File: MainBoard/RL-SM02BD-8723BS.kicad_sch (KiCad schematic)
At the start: 20 parts, among them U401 RTL8723BS(ComboModule)

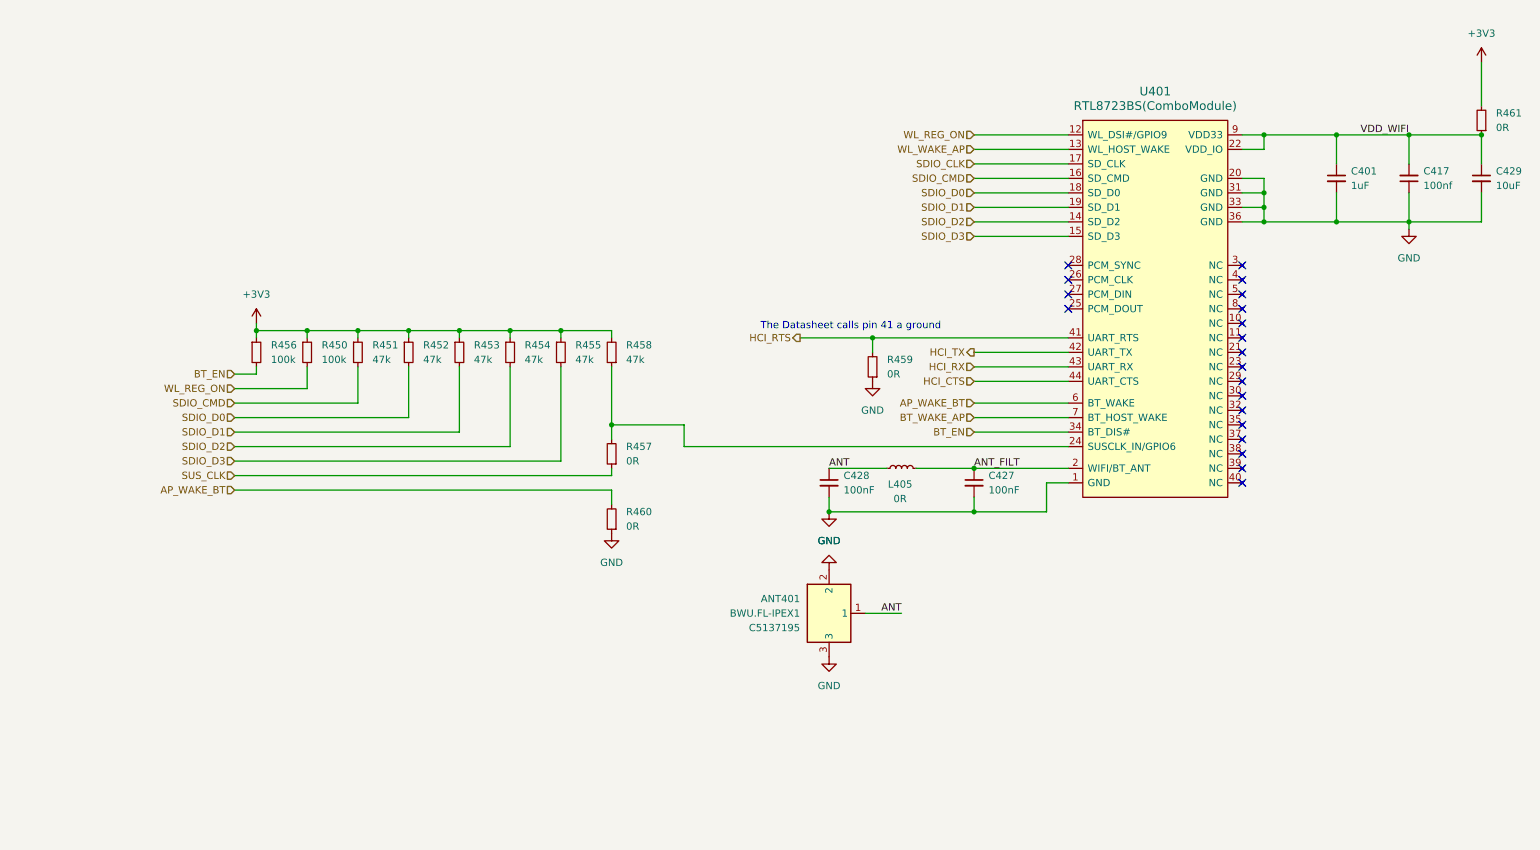
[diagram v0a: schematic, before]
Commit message: Submit for fab rev 2
Signed-off-by: Connor Rigby <connorr@hey.com>
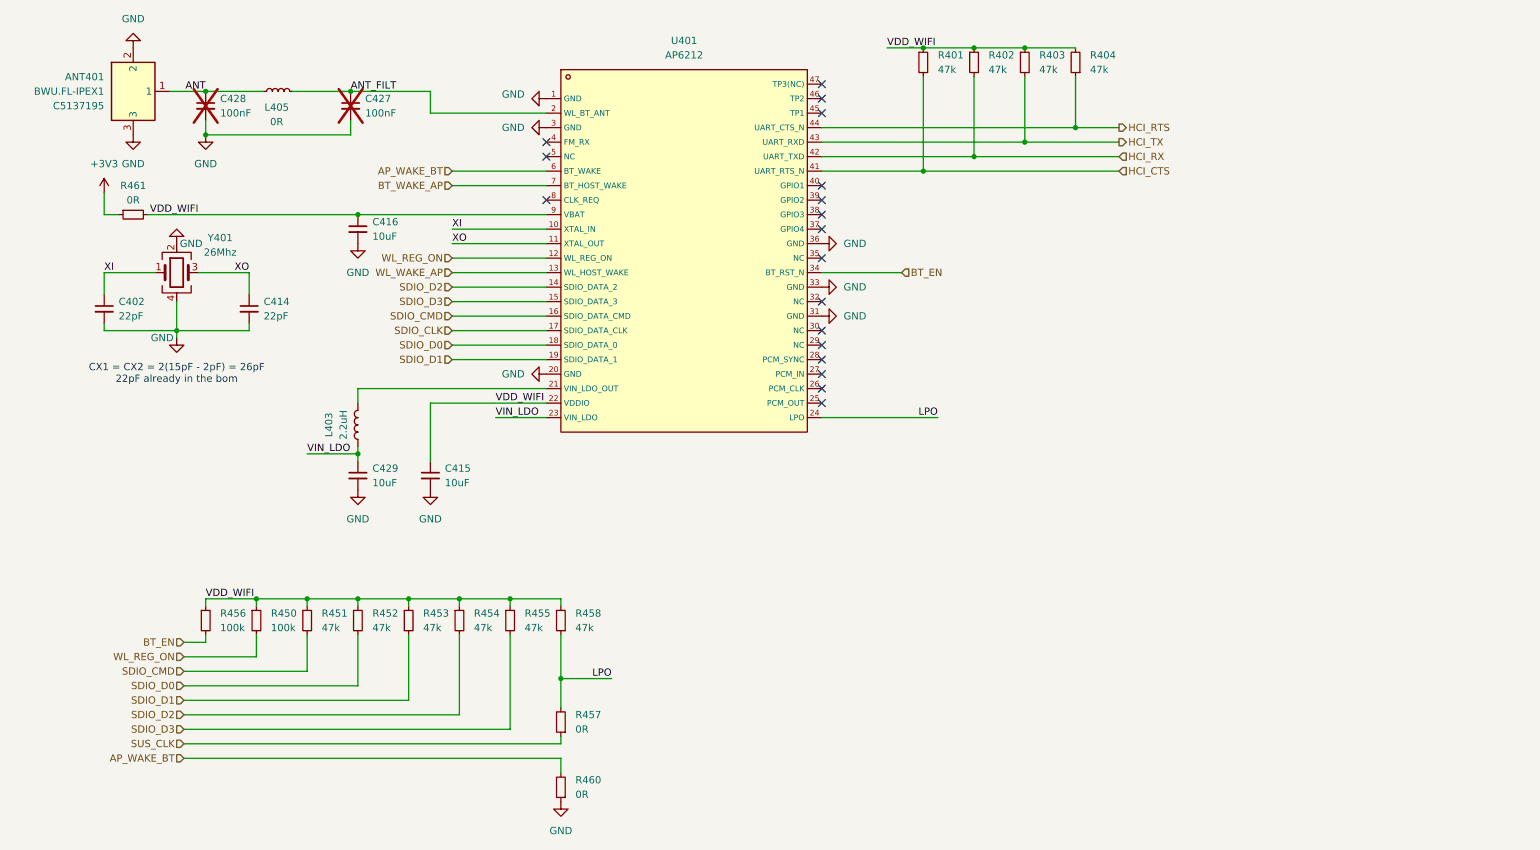
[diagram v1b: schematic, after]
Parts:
- removed C401: 1uF, Resistor_SMD:R_0402_1005Metric, symbol Device:C_Small
- removed C417: 100nf, Capacitor_SMD:C_0402_1005Metric, symbol Device:C_Small
- removed R459: 0R, Resistor_SMD:R_0402_1005Metric, symbol Device:R_Small
- removed U401: RTL8723BS(ComboModule), Module_WiFi_BT:RL-SM02BD(RTL8723BS), symbol Module_WiFi_BT:RTL8723BS(ComboModule)
- added C402, C414: 22pF, Capacitor_SMD:C_0402_1005Metric, symbol Device:C_Small
- added C415, C416: 10uF, Capacitor_SMD:C_0603_1608Metric, symbol Device:C_Small
- added L403: 2.2uH, Inductor_SMD:L_0603_1608Metric, symbol Device:L
- added R401, R402, R403, R404: 47k, Resistor_SMD:R_0402_1005Metric, symbol Device:R_Small
- added U401: AP6212, Module_WiFi_BT:QFN-44_L12.0-W12.0-P0.90-TL_AP6212, symbol Module_WiFi_BT:AP6212
- added Y401: 26Mhz, Crystal:Crystal_SMD_3225-4Pin_3.2x2.5mm, symbol Device:Crystal_GND24
- C427, C428: now not fitted; now left out of the parts list
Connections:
- net +3V3: now also R461.1; no longer R450.1, R451.1, R452.1, R453.1, R454.1, R455.1, R456.1, R458.2, R461.2
- net ANT_FILT: now also U401.2 (WL_BT_ANT)
- net AP_WAKE_BT: now also U401.6 (BT_WAKE)
- net BT_EN: now also U401.34 (BT_RST_N)
- net BT_WAKE_AP: now also U401.7 (BT_HOST_WAKE)
- net GND: now also C402.2, C414.2, C415.2, C416.2, U401.1 (GND), U401.20 (GND), U401.3 (GND), U401.31 (GND), U401.33 (GND), U401.36 (GND), Y401.2, Y401.4
- net HCI_CTS: now also R401.2, U401.41 (UART_RTS_N)
- net HCI_RTS: now also R404.1, U401.44 (UART_CTS_N)
- net HCI_RX: now also R402.2, U401.42 (UART_TXD)
- net HCI_TX: now also R403.2, U401.43 (UART_RXD)
- net SDIO_CLK: now also U401.17 (SDIO_DATA_CLK)
- net SDIO_CMD: now also U401.16 (SDIO_DATA_CMD)
- net SDIO_D0: now also U401.18 (SDIO_DATA_0)
- net SDIO_D1: now also U401.19 (SDIO_DATA_1)
- net SDIO_D2: now also U401.14 (SDIO_DATA_2)
- net SDIO_D3: now also U401.15 (SDIO_DATA_3)
- net VDD_WIFI: now also R450.1, R451.1, R452.1, R453.1, R454.1, R455.1, R456.1, R458.2, R461.2, C415.1, C416.1, R401.1, R402.1, R403.1, R404.2, U401.22 (VDDIO), U401.9 (VBAT); no longer C429.1, R461.1
- net WL_REG_ON: now also U401.12 (WL_REG_ON)
- net WL_WAKE_AP: now also U401.13 (WL_HOST_WAKE)
- net LPO: now reaches R457.2, R458.1
- net LPO: now also U401.24 (LPO)
- new net: L403.2, U401.21 (VIN_LDO_OUT)
- new net VIN_LDO: C429.1, L403.1, U401.23 (VIN_LDO)
- new net XI: C402.1, U401.10 (XTAL_IN), Y401.1
- new net XO: C414.1, U401.11 (XTAL_OUT), Y401.3
- no-connect marks 20 -> 18
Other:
- note added: "CX1 = CX2 = 2(15pF - 2pF) = 26pF 22pF already in the bom"
- note removed: "The Datasheet calls pin 41 a ground"
- moved on the sheet: ANT401, C429, L405, R450, R451, R452, R453, R454, R455, R456, R457, R458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
